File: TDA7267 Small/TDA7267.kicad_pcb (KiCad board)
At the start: 2 copper layers, 43 x 39 mm, 18 parts, among them U1 TDA7267

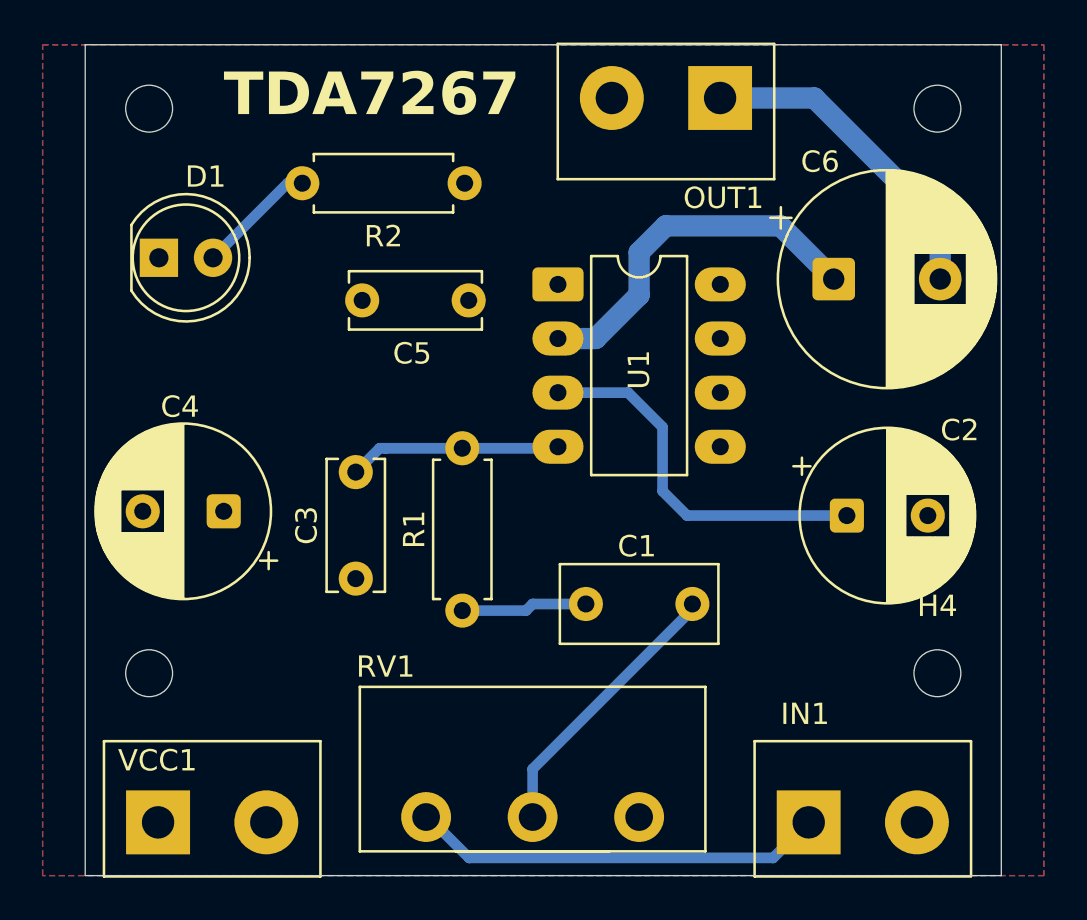
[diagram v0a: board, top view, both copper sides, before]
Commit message: More stuff
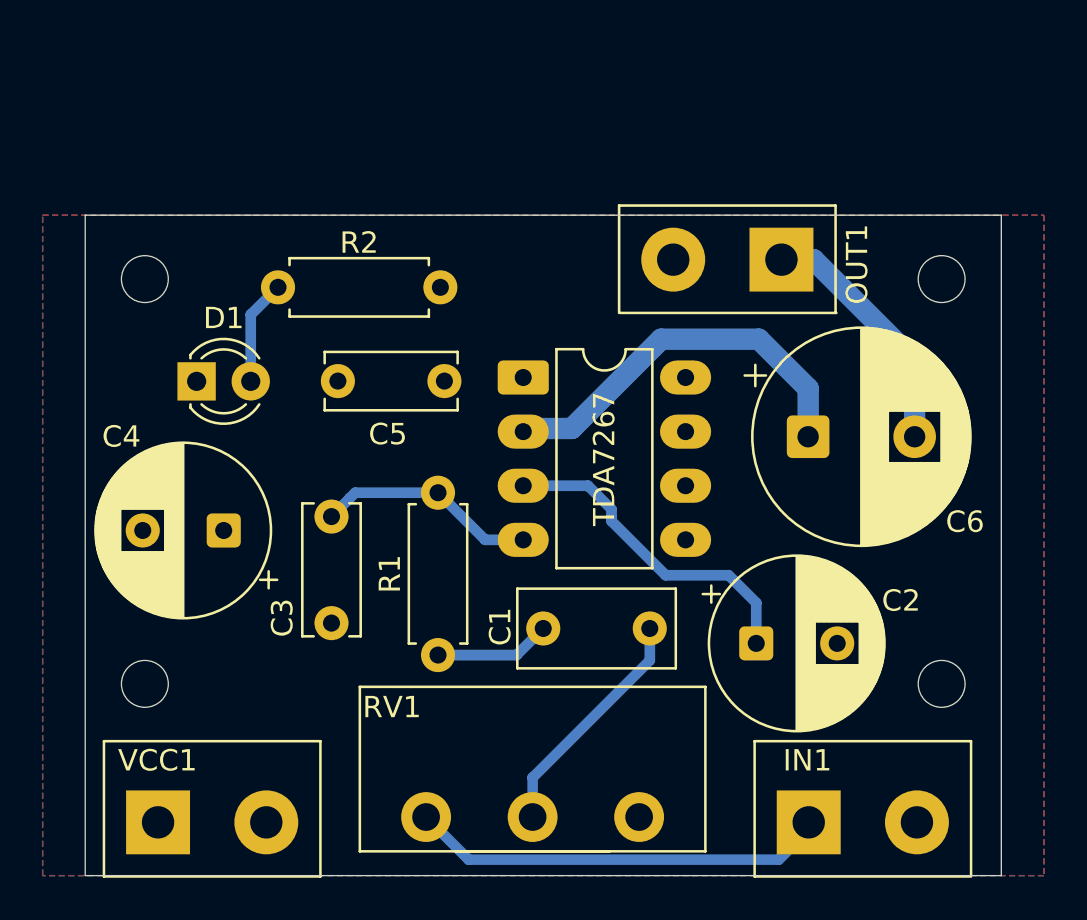
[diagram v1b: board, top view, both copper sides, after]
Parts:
- D1: footprint LED_THT:LED_D5.0mm -> LED_THT:LED_D3.0mm
- moved OUT1 8.12 mm to (161.7, 88.6)
- moved H1 8.00 mm to (131.8, 89.5)
- moved H2 8.00 mm to (169.2, 89.5)
- moved C6 7.50 mm to (162.9, 96.9)
- moved C2 7.35 mm to (160.5, 106.6)
- moved D1 6.06 mm to (134.2, 94.3)
- moved R2 5.02 mm to (138.1, 89.9)
- moved TDA7267 4.66 mm to (149.6, 94.1)
- moved C5 3.96 mm to (140.9, 94.3)
- moved C3 2.38 mm to (140.6, 105.6)
- moved R1 2.38 mm to (145.6, 107.1)
- moved C1 2.31 mm to (155.5, 105.9)
- moved C4 0.90 mm to (135.5, 101.3)
- moved H3 0.54 mm to (131.8, 108.5)
- moved H4 0.54 mm to (169.2, 108.5)
- renumbered U1 to TDA7267
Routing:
- net Net-(OUT1-Pin_1): track 15.4 -> 11.8 mm
- net Net-(U1-SRV): track 17.7 -> 15.4 mm
- net Net-(C1-Pad1): track 13.1 -> 11.1 mm
- net Net-(U1-Out): track 17.3 -> 18.4 mm
- net Net-(D1-A): track 5.64 -> 4.94 mm
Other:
- board size 43 x 39 mm -> 43 x 31 mm
- board text removed: "TDA7267"
